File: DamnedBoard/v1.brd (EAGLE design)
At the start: 39 x 16.5 mm, 17 parts, among them U1 EFM32ZG108, U2 MAX44009EDT+T21-0490D-M

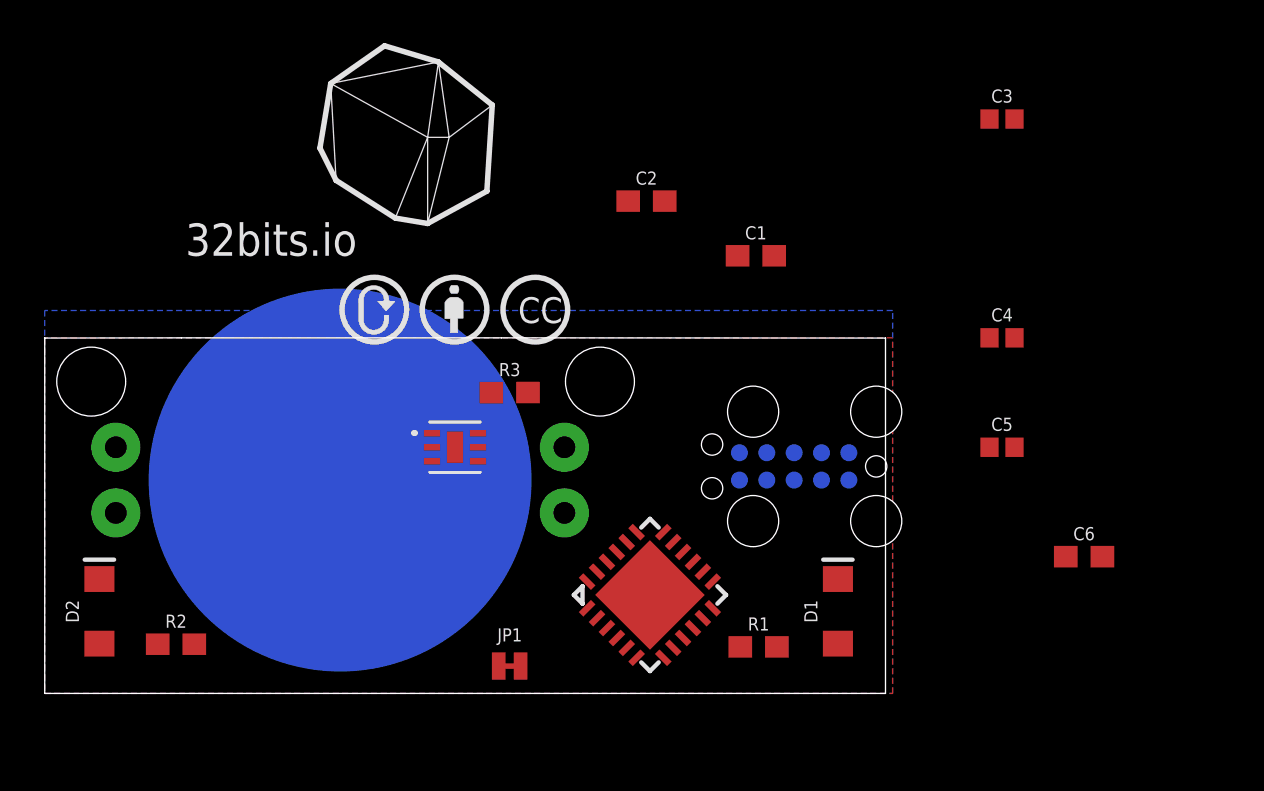
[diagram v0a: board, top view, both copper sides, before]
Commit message: OSH Parkifying layout.
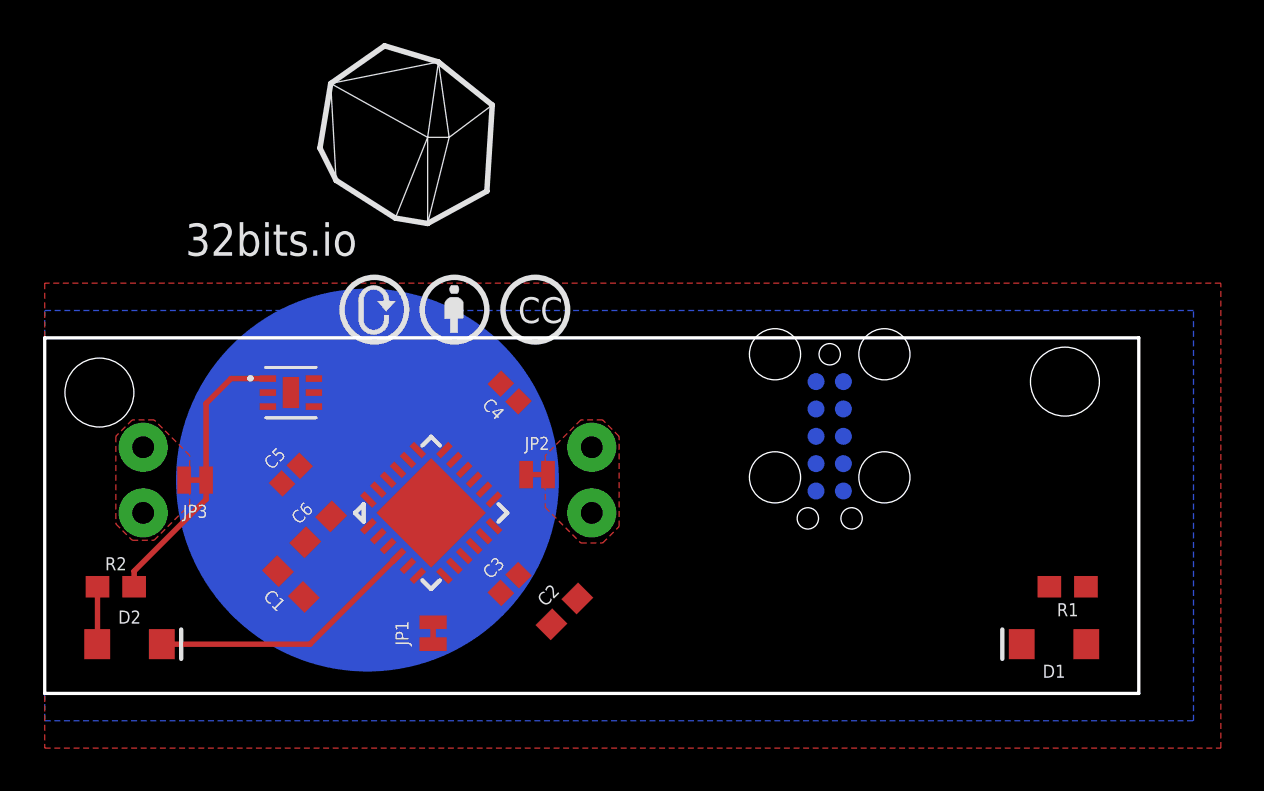
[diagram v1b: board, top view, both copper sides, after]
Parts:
- removed R3: 0, SparkFun-Resistors:0603
- added JP2, JP3: JUMPER-SMT_2_NC_TRACE_NO-SILK, SparkFun-Jumpers:SMT-JUMPER_2_NC_TRACE_NO-SILK
- moved C6 35.6 mm to (12.7, 7.62), turned to 45 degrees
- moved C5 33.0 mm to (11.4, 10.2), turned to 45 degrees
- moved C3 31.4 mm to (21.6, 5.08), turned to 45 degrees
- moved C1 26.4 mm to (11.4, 5.08), turned to 135 degrees
- moved C4 23.0 mm to (21.6, 14.0), turned to 135 degrees
- moved C2 19.4 mm to (24.1, 3.81), turned to 45 degrees
- moved R1 14.6 mm to (47.5, 4.95), turned to 180 degrees
- moved U1 10.9 mm to (14.4, 8.38)
- moved D1 10.1 mm to (46.9, 2.29), turned to 180 degrees
- moved U2 8.03 mm to (11.4, 14.0)
- moved JP1 3.87 mm to (18.0, 2.79), turned to 90 degrees
- moved R2 3.86 mm to (3.30, 4.95)
- moved TC1 2.16 mm to (36.4, 11.9), turned to 270 degrees
- moved D2 2.07 mm to (3.94, 2.29), turned to 0 degrees
- moved G1 1.27 mm to (25.4, 11.4)
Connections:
- removed net N$1: G1.P$1, G1.P$2, G1.P$3, G1.P$4, R3.2
- new net +L: G1.P$1, G1.P$2, JP2.2
- new net +R: G1.P$3, G1.P$4, JP3.2
- net VCC: now also JP2.1, JP3.1; no longer R3.1
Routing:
- net PC1: track 0.00 -> 12.7 mm
- net VCC: track 0.00 -> 12.4 mm
- net N$2: track 0.00 -> 2.67 mm
- added copper zone on layer 1, net +L
- added copper zone on layer 1, net +R
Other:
- board size 39 x 16.5 mm -> 50.8 x 16.5 mm
